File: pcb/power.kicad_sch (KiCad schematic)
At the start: 9 parts, among them U5 L7805, U6 L7805

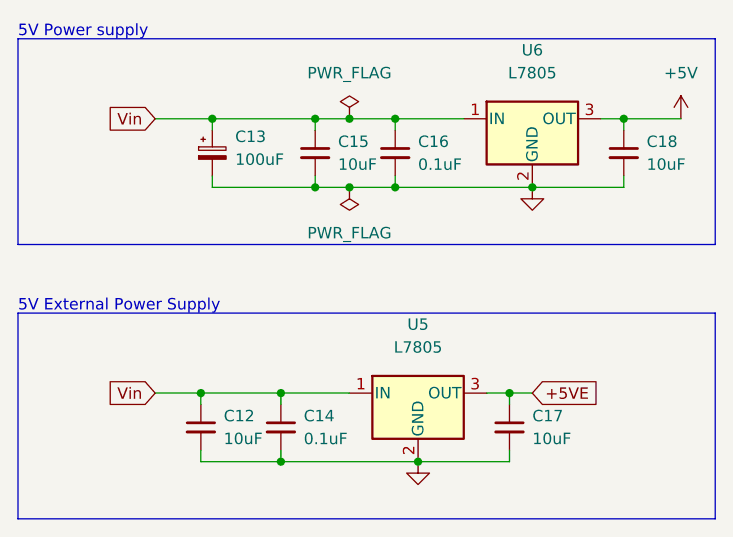
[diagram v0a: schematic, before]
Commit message: CI/CD Changes
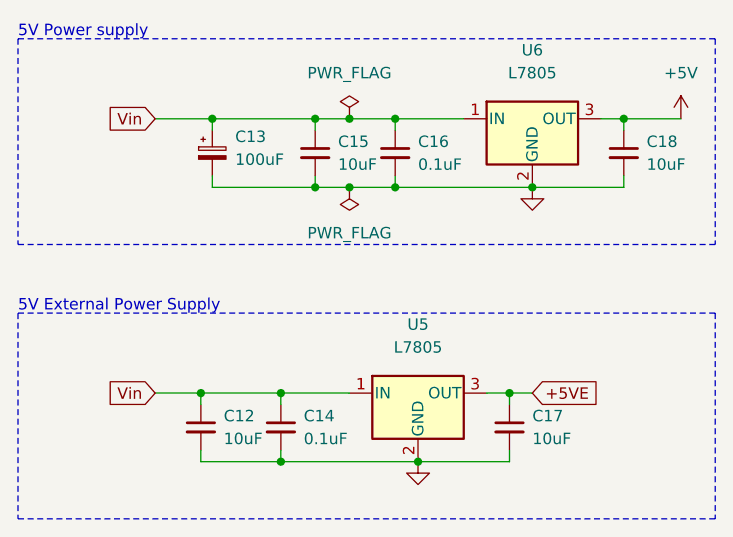
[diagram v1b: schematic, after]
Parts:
- C12, C15, C17, C18: Spice_Model 10u -> (none); Spice_Netlist_Enabled N -> (none); Spice_Primitive C -> (none)
- C14, C16: Spice_Model 0.1u -> (none); Spice_Netlist_Enabled N -> (none); Spice_Primitive C -> (none)
